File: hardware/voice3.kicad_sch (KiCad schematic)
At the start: 30 parts, among them IC1 LM13700, U12 MCP4922-ESL, U9 SSI2144

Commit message: hardware: proper production files for JLCPCB
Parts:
- C75, C76, C77: LCSC C5299898 -> C115056
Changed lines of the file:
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@@
       (effects (font (size 1.524 1.524)))
     )
-    (property "LCSC" "C5299898" (at 114.3 87.63 0)
+    (property "LCSC" "C115056" (at 114.3 87.63 0)
       (effects (font (size 1.27 1.27)) hide)
     )
@@
       (effects (font (size 1.524 1.524)))
     )
-    (property "LCSC" "C5299898" (at 114.3 95.25 0)
+    (property "LCSC" "C115056" (at 114.3 95.25 0)
       (effects (font (size 1.27 1.27)) hide)
     )
@@
       (effects (font (size 1.524 1.524)))
     )
-    (property "LCSC" "C5299898" (at 109.22 102.87 0)
+    (property "LCSC" "C115056" (at 109.22 102.87 0)
       (effects (font (size 1.27 1.27)) hide)
     )

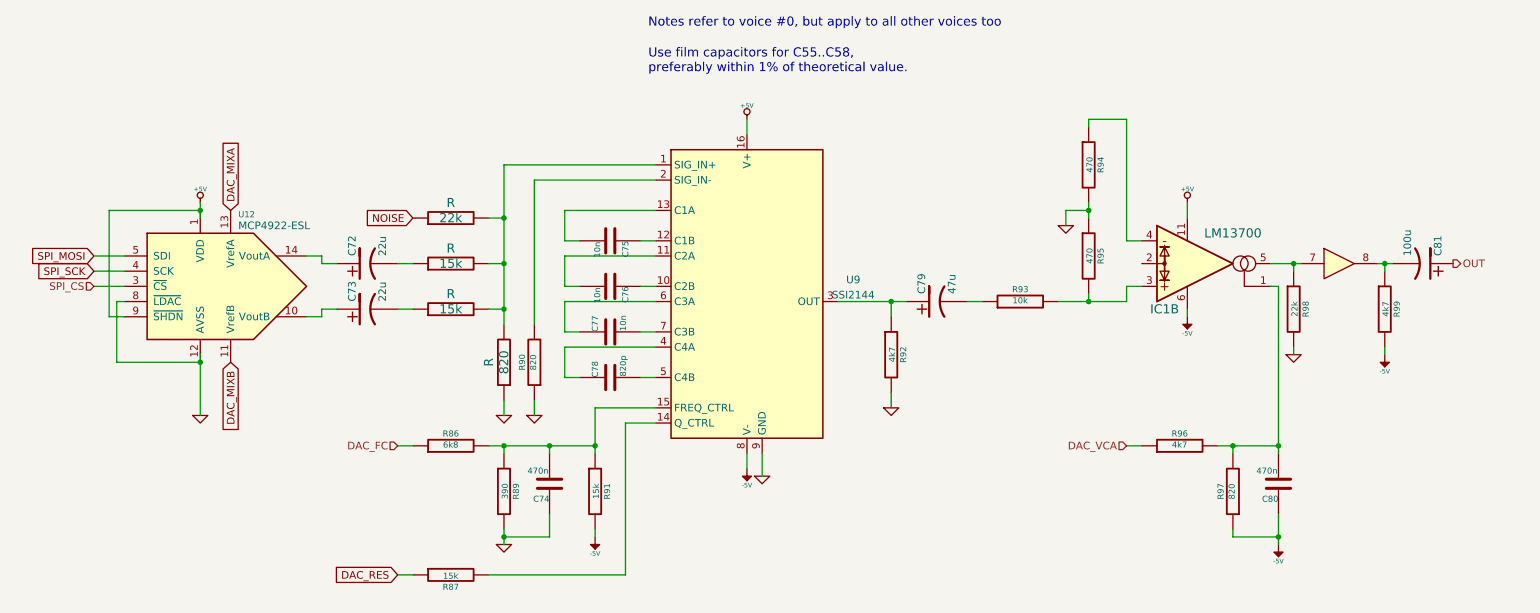
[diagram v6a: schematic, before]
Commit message: hardware: Schematics rework by Guimli
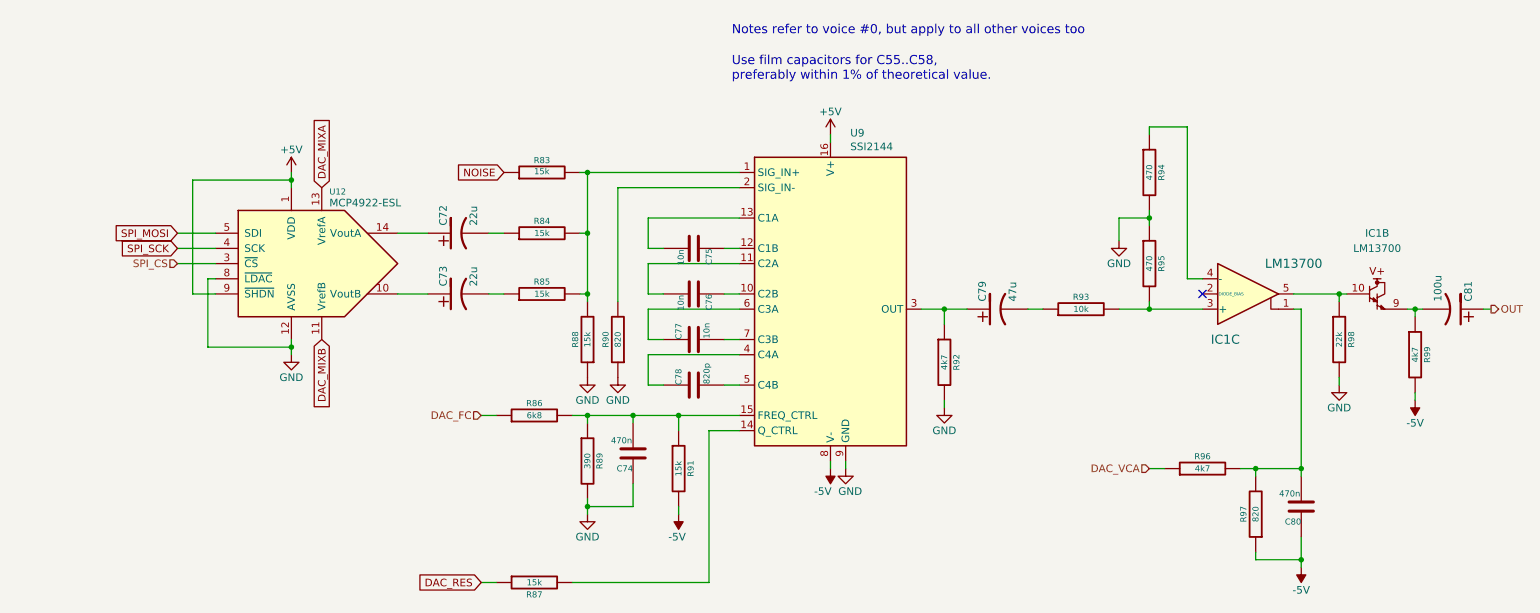
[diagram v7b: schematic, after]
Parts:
- added unit 2 of IC1
- C72, C73, C79, C81: symbol overcycler2-rescue:CP1 -> Additional:CP
- C74, C75, C76, C77, C78, C80: symbol overcycler2-rescue:C -> Additional:C
- IC1: symbol overcycler2-rescue:LM13700 -> Amplifier_Operational:LM13700
- R83, R84, R85, R88: renamed from R; footprint ~ -> Resistor_SMD:R_0805_2012Metric; symbol overcycler2-rescue:R -> Additional:R
- R86, R87, R89, R90, R91, R92, R93, R94, R95, R96, R97, R98, R99: symbol overcycler2-rescue:R -> Additional:R
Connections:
- net +5V: no longer IC1.11 (V+)
- net -5V: no longer IC1.6 (V-)
- net at IC1.5, R98.1: now also IC1.10; no longer IC1.7 (buffer_in)
- net at C81.2, R99.1: now also IC1.9; no longer IC1.8 (buffer_out)
- no-connect marks 0 -> 1
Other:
- moved on the sheet: C72, C73, C74, C75, C76, C77, C78, C79, C80, C81, R83, R84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
